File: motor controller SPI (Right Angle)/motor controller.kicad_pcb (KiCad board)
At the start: 2 copper layers, 38 x 18 mm, 27 parts, among them IC1 MA702, IC2 MC33926PNB, IC3 LP38690SD-ADJ_NOPB, J1 Conn_01x06_Male, J2 Conn_01x06_Male, J3 Conn_01x04_Male, M1 Motor_DC, U1 STM32L432KCUx, Y1 32mhz

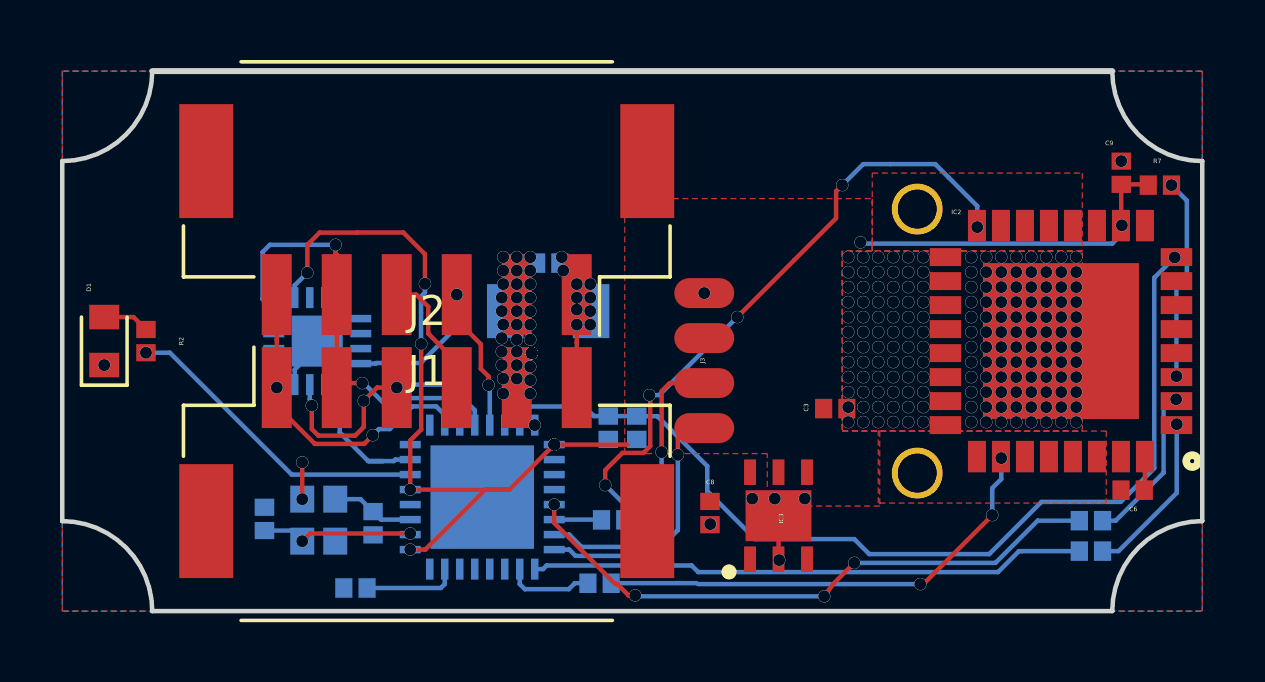
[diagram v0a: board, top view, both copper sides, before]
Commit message: Updated footprints
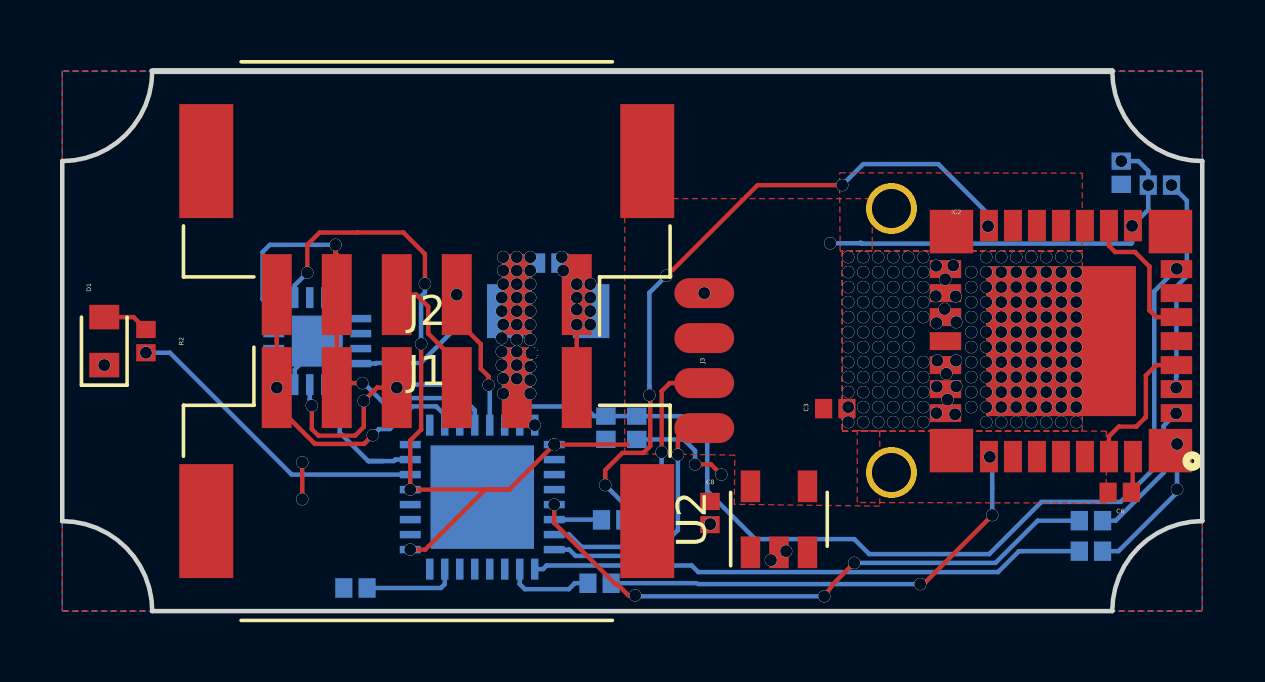
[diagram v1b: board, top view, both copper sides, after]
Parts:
- removed C1, C2: 10pF, Capacitor_SMD:C_0402_1005Metric
- removed IC3: LP38690SD-ADJ_NOPB, LP38690SD-ADJ_NOPB:SON95P300X300X80-7N
- removed Y1: 32mhz, Crystal:Crystal_SMD_2016-4Pin_2.0x1.6mm
- added U2: MIC5501-3.0YM5, Package_TO_SOT_SMD:SOT-23-5, F.Cu at (23.9, 14.9)
- C9, R7: moved to B.Cu
- moved M1 0.86 mm to (27.6, 8.98)
- moved C6 0.44 mm to (35.2, 14.0)
- moved C5 0.08 mm to (18.1, 11.9)
- turned C9 to 270 degrees
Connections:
- IC1 pad 1: Net-(IC1-Pad1) -> (no net)
- IC1 pad 10: Net-(IC1-Pad10) -> (no net)
- IC1 pad 11: Net-(IC1-Pad11) -> (no net)
- IC1 pad 14: Net-(IC1-Pad14) -> (no net)
- IC1 pad 15: Net-(IC1-Pad15) -> (no net)
- IC1 pad 16: Net-(IC1-Pad16) -> (no net)
- IC1 pad 2: Net-(IC1-Pad2) -> (no net)
- IC1 pad 3: Net-(IC1-Pad3) -> (no net)
- IC1 pad 6: Net-(IC1-Pad6) -> (no net)
- IC1 pad 9: Net-(IC1-Pad9) -> (no net)
- IC2 pad 17: Net-(IC2-Pad17) -> (no net)
- IC2 pad 21: Net-(IC2-Pad21) -> (no net)
- IC2 pad 25: Net-(IC2-Pad25) -> (no net)
- IC2 pad 5: Net-(IC2-Pad5) -> (no net)
- IC2 pad 7: Net-(IC2-Pad7) -> (no net)
- IC2 pad 9: Net-(IC2-Pad9) -> (no net)
- U1 pad 15: Net-(U1-Pad15) -> (no net)
- U1 pad 18: Net-(U1-Pad18) -> (no net)
- U1 pad 19: Net-(U1-Pad19) -> (no net)
- U1 pad 2: Net-(C1-Pad1) -> (no net)
- U1 pad 20: Net-(U1-Pad20) -> (no net)
- U1 pad 27: Net-(U1-Pad27) -> (no net)
- U1 pad 28: Net-(U1-Pad28) -> (no net)
- U1 pad 29: Net-(U1-Pad29) -> (no net)
- U1 pad 3: Net-(C2-Pad2) -> (no net)
- U1 pad 30: Net-(U1-Pad30) -> (no net)
- U1 pad 4: Net-(U1-Pad4) -> (no net)
- U1 pad 8: Net-(U1-Pad8) -> (no net)
- U1 pad 9: Net-(U1-Pad9) -> (no net)
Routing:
- net +BATT: track 3.10 -> 12.6 mm
- net Net-(C1-Pad1): track 5.15 -> 0.00 mm, vias 2 -> 0
- net Net-(C2-Pad2): track 2.78 -> 0.00 mm
- net +3V3: track 37.8 -> 40.2 mm, vias 9 -> 11
- net GND: track 9.20 -> 11.3 mm, vias 213 -> 224
- net Net-(IC2-Pad16): track 21.4 -> 23.1 mm
- net Net-(IC2-Pad2): track 5.52 -> 4.85 mm
- net Net-(IC2-Pad1): track 5.57 -> 4.91 mm, vias 1 -> 2
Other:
- rule via_min_size: 0.4 -> 0.2

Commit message: Push to new server
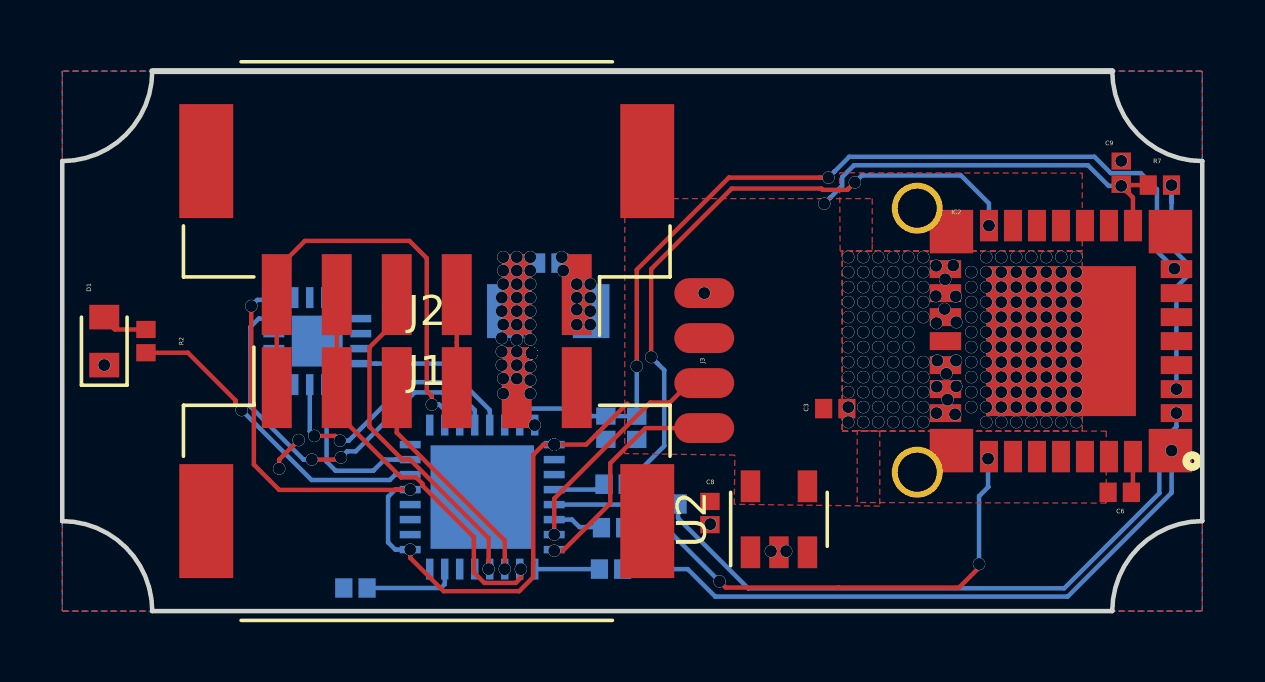
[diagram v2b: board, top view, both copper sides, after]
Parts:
- C9, R7: moved to F.Cu
- moved R5 16.0 mm to (18.3, 16.6)
- moved R6 14.2 mm to (20.1, 14.4)
- moved R8 1.90 mm to (18.4, 15.2)
- moved R9 1.19 mm to (18.4, 13.8)
- moved M1 0.86 mm to (28.5, 8.97)
- turned C9 to 90 degrees
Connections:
- J1 pad 3: MOSI -> Net-(J1-Pad3)
- J1 pad 4: Net-(J1-Pad4) -> CommsMOSI
- J1 pad 5: SCK -> CommsSCK
- J2 pad 2: SCK -> CommsSCK
- J2 pad 3: MISO -> CommsMISO
- J2 pad 4: Net-(J1-Pad4) -> Net-(J1-Pad3)
- U1 pad 20: (no net) -> D2
- U1 pad 22: D2 -> D1
- U1 pad 26: D1 -> CommsSCK
- U1 pad 27: (no net) -> CommsMISO
- U1 pad 28: (no net) -> CommsMOSI
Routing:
- net IN1: track 20.3 -> 3.36 mm, vias 4 -> 0
- net Net-(IC2-Pad2): track 4.85 -> 21.7 mm
- net Net-(IC2-Pad1): track 4.91 -> 21.5 mm, vias 2 -> 1
- net IN2: track 18.6 -> 2.16 mm
- net CommsSCK: track 0.00 -> 13.6 mm, vias 0 -> 1
- net +BATT: track 12.6 -> 0.00 mm
- net CommsMOSI: track 0.00 -> 11.3 mm, vias 0 -> 1
- net GND: track 11.3 -> 1.22 mm, vias 224 -> 223
- net CommsMISO: track 0.00 -> 8.39 mm, vias 0 -> 1
- net CS: track 10.8 -> 15.5 mm, vias 2 -> 1
- net Net-(J1-Pad4): track 4.31 -> 0.00 mm
- net MOSI: track 9.59 -> 5.44 mm, vias 2 -> 0
- net Net-(J1-Pad3): track 0.00 -> 3.10 mm
- net SWDIO: track 10.0 -> 7.79 mm
- net SCK: track 14.9 -> 12.9 mm
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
